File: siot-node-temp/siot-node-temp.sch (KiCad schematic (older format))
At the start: 9 parts, among them J1 xConnect_smd, J2 Conn_01x03, J3 Conn_01x03, J4 xConnect_smd, U1 ADP7142AUJZ-3.3

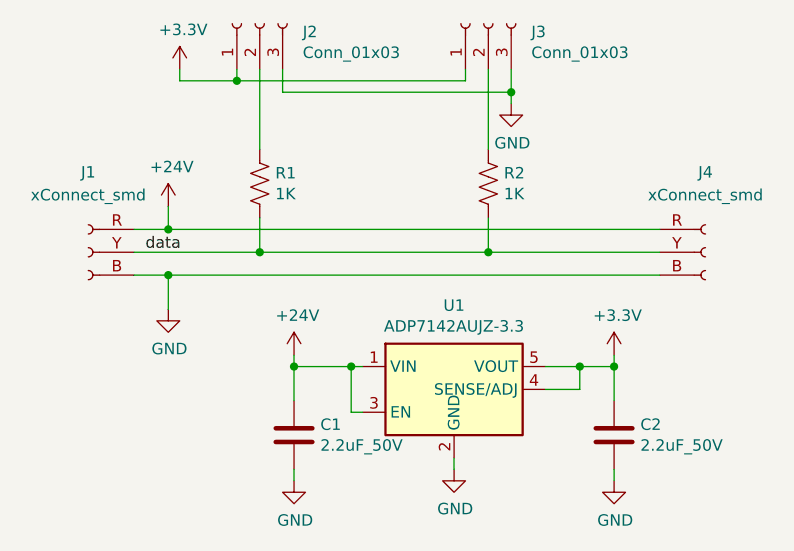
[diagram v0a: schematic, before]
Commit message: updates
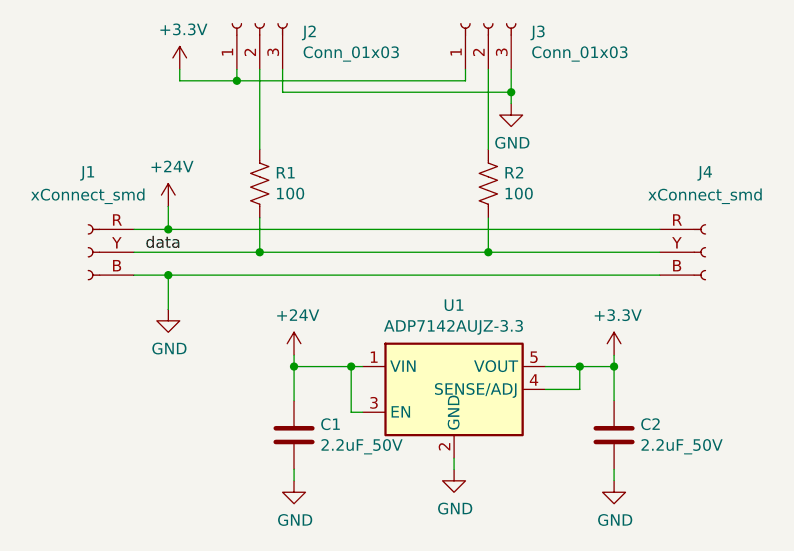
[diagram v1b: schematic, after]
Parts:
- R1, R2: value 1K -> 100
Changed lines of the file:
@@
 P 4800 3200
 F 0 "R1" H 4868 3246 50  0000 L CNN
-F 1 "1K" H 4868 3155 50  0000 L CNN
+F 1 "100" H 4868 3155 50  0000 L CNN
 F 2 "Resistor_SMD:R_0603_1608Metric" V 4840 3190 50  0001 C CNN
 F 3 "~" H 4800 3200 50  0001 C CNN
@@
 P 5800 3200
 F 0 "R2" H 5868 3246 50  0000 L CNN
-F 1 "1K" H 5868 3155 50  0000 L CNN
+F 1 "100" H 5868 3155 50  0000 L CNN
 F 2 "Resistor_SMD:R_0603_1608Metric" V 5840 3190 50  0001 C CNN
 F 3 "~" H 5800 3200 50  0001 C CNN

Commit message: temp node tweaks
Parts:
- U1: value ADP7142AUJZ-3.3 -> ADP7142AUJZ-5.0; symbol bec-power:ADP7142AUJZ-3.3 -> bec-power:ADP7142AUJZ-5.0; MPN ADP7142AUJZ-3.3 -> ADP7142AUJZ-5.0
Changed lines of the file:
@@
 $EndComp
 $Comp
-L bec-power:ADP7142AUJZ-3.3 U1
+L bec-power:ADP7142AUJZ-5.0 U1
 U 1 1 5D68AE2A
 P 5650 4100
 F 0 "U1" H 5650 4467 50  0000 C CNN
-F 1 "ADP7142AUJZ-3.3" H 5650 4376 50  0000 C CNN
+F 1 "ADP7142AUJZ-5.0" H 5650 4376 50  0000 C CNN
 F 2 "Package_TO_SOT_SMD:TSOT-23-5" H 5650 3700 50  0001 C CIN
 F 3 "https://www.analog.com/media/en/technical-documentation/data-sheets/ADP7142.pdf" H 5650 3600 50  0001 C CNN
-F 4 "ADP7142AUJZ-3.3" H 5650 4100 50  0001 C CNN "MPN"
+F 4 "ADP7142AUJZ-5.0" H 5650 4100 50  0001 C CNN "MPN"
 F 5 "Analog Devices" H 5650 4100 50  0001 C CNN "Manufacturer"
 	1    5650 4100

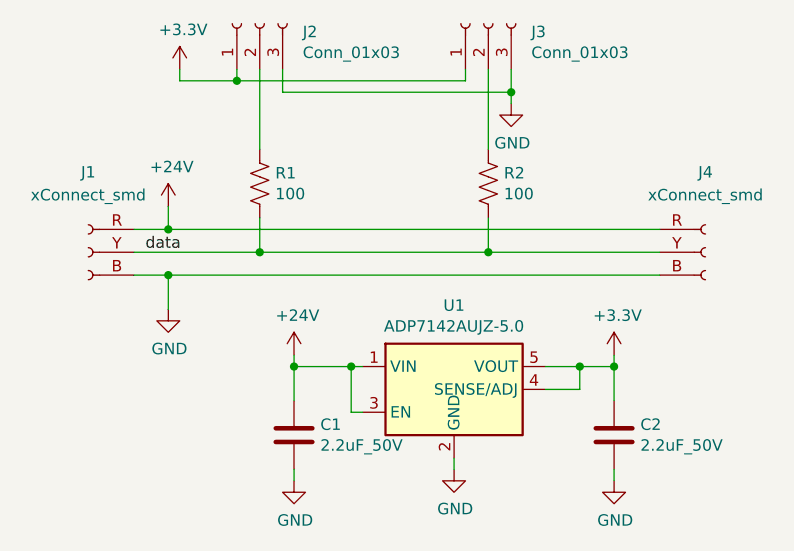
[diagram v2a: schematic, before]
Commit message: updates
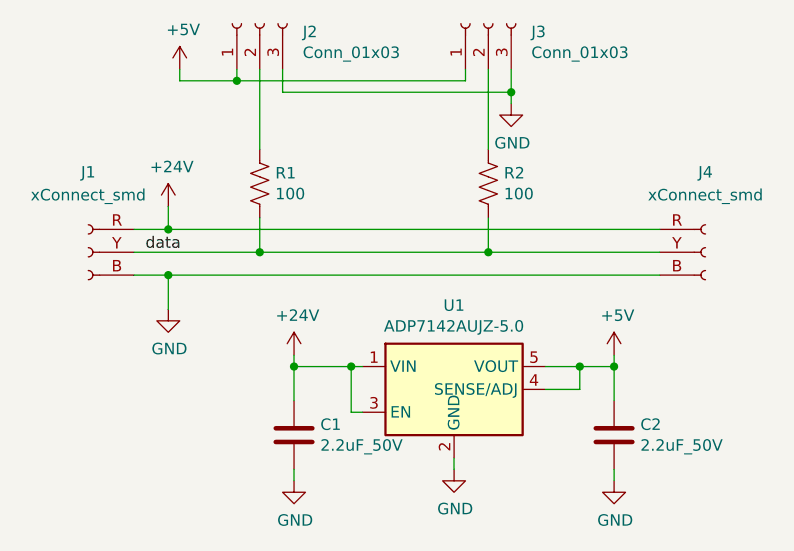
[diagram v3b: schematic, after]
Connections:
- net +3V3 renamed +5V
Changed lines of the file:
@@
 Wire Wire Line
 	6200 4000 6350 4000
-$Comp
-L power:+3.3V #PWR0101
-U 1 1 5D693774
-P 6350 3950
-F 0 "#PWR0101" H 6350 3800 50  0001 C CNN
-F 1 "+3.3V" H 6365 4123 50  0000 C CNN
-F 2 "" H 6350 3950 50  0001 C CNN
-F 3 "" H 6350 3950 50  0001 C CNN
-	1    6350 3950
-	1    0    0    -1
-$EndComp
-$Comp
-L power:+3.3V #PWR0102
-U 1 1 5D693C5B
-P 4450 2700
-F 0 "#PWR0102" H 4450 2550 50  0001 C CNN
-F 1 "+3.3V" H 4465 2873 50  0000 C CNN
-F 2 "" H 4450 2700 50  0001 C CNN
-F 3 "" H 4450 2700 50  0001 C CNN
-	1    4450 2700
-	1    0    0    -1
-$EndComp
 Wire Wire Line
 	5200 4000 5200 4200
@@
 Wire Wire Line
 	5200 4000 5250 4000
+$Comp
+L power:+5V #PWR?
+U 1 1 5DCE3829
+P 4450 2700
+F 0 "#PWR?" H 4450 2550 50  0001 C CNN
+F 1 "+5V" H 4465 2873 50  0000 C CNN
+F 2 "" H 4450 2700 50  0001 C CNN
+F 3 "" H 4450 2700 50  0001 C CNN
+	1    4450 2700
+	1    0    0    -1
+$EndComp
+$Comp
+L power:+5V #PWR?
+U 1 1 5DCE3E5A
+P 6350 3950
+F 0 "#PWR?" H 6350 3800 50  0001 C CNN
+F 1 "+5V" H 6365 4123 50  0000 C CNN
+F 2 "" H 6350 3950 50  0001 C CNN
+F 3 "" H 6350 3950 50  0001 C CNN
+	1    6350 3950
+	1    0    0    -1
+$EndComp
 $EndSCHEMATC
